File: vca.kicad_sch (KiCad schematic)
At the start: 29 parts, among them Q1 BC549C, Q2 BC549C, Q3 BC549C, Q4 BC549C, Q5 BC549C, Q6 BC549C, Q7 BC549C, Q8 BC549C, Q9 BC549C, U1 NE5532

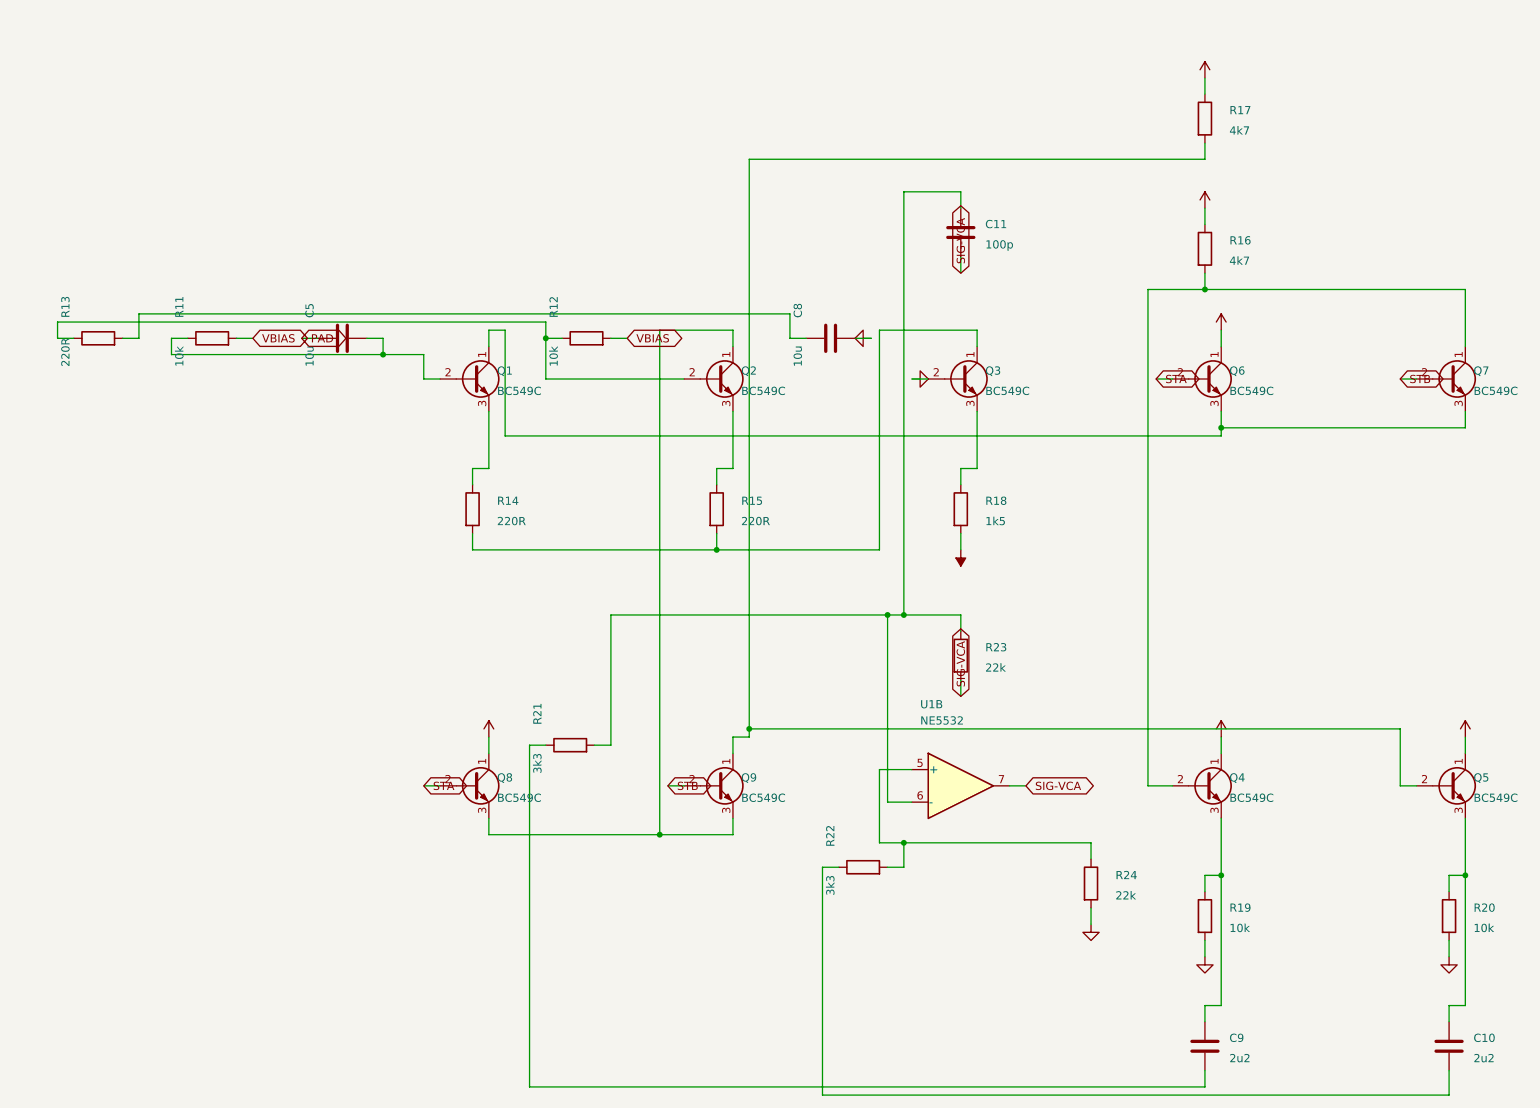
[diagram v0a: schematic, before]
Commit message: add Docs & fix name & all the other shit
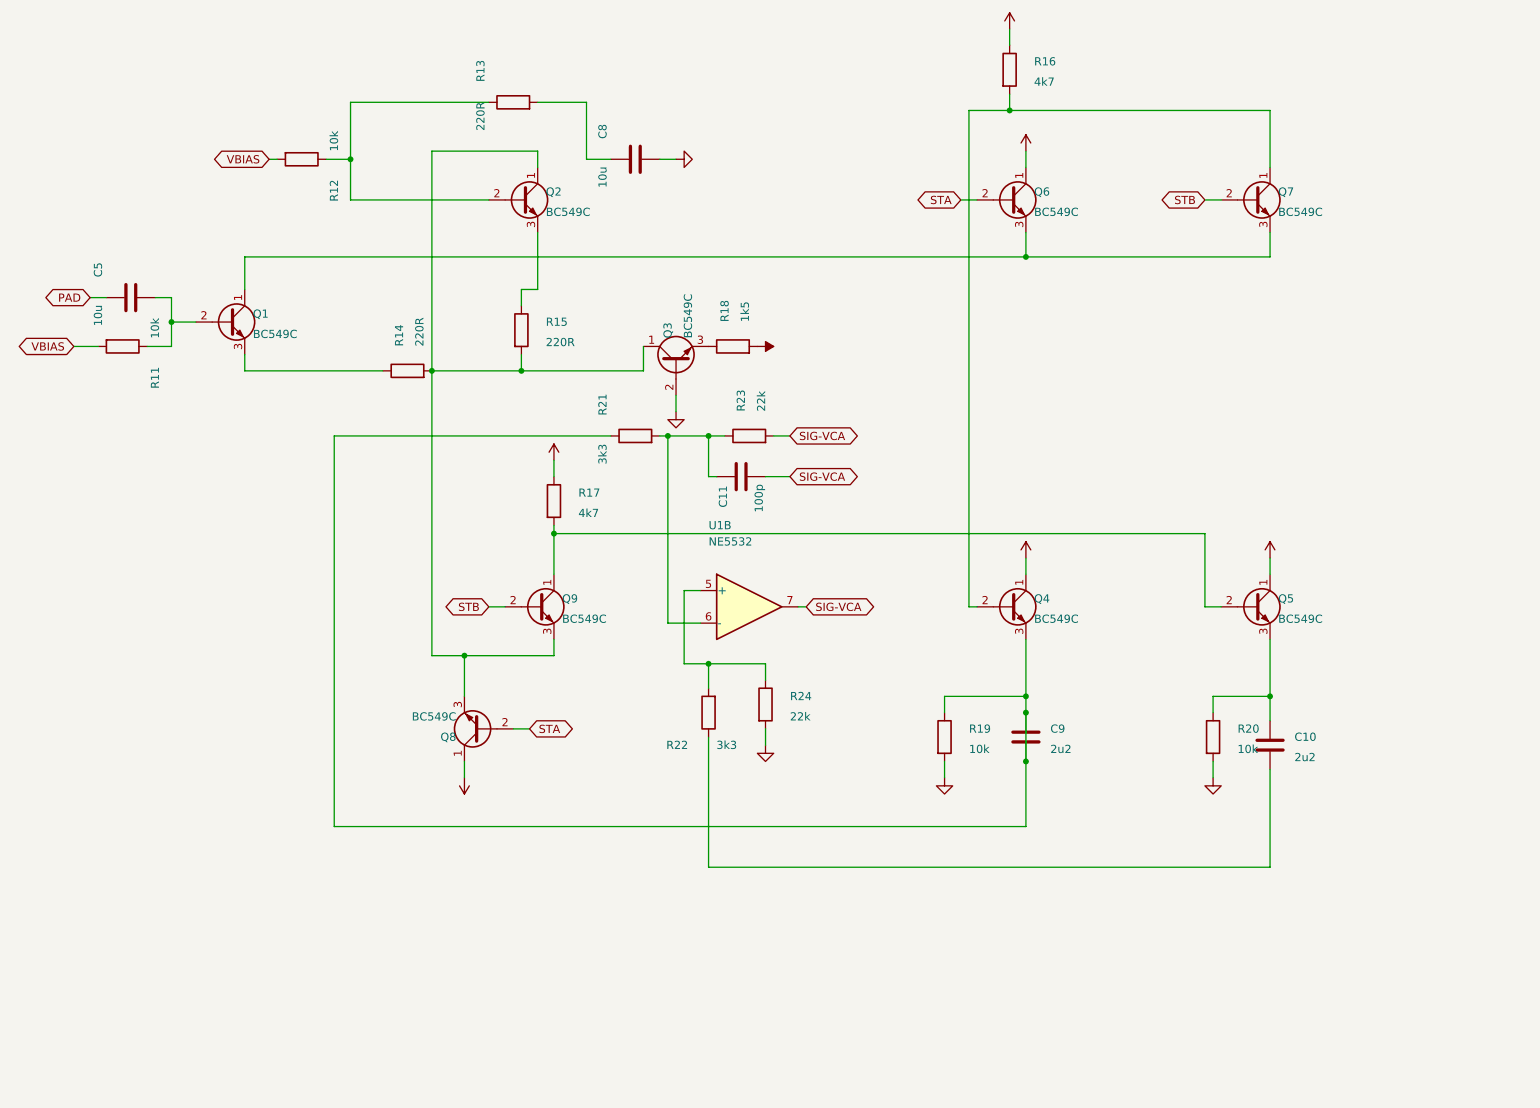
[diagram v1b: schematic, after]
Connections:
- net at Q3.1 (C), R14.2, R15.2: now also Q2.1 (C), Q8.3 (E), Q9.3 (E)
- net at C9.1, Q4.3 (E), R19.1: now also C9.2, R21.1
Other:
- company: Steer 500 -> UTS Mini Mixing Desk
- title: Steer 500 - 3 VCA -> UTS Mini Mixing Desk - Compressor
- moved on the sheet: C10, C11, C5, C8, C9, Q1, Q2, Q3, Q4, Q5, Q6, Q7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
